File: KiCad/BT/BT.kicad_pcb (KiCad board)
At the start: 4 copper layers, 13.8 x 31.5 mm, 54 parts, among them J1 UJC-HP-3-SMT-TR, J2 2328702-8, J3 Conn_01x05, SW1 Val**, U1 QFN40P120X130X45-6N, U2 SON95P300X300X100-7N-D, U3 STM6601CQ2BDM6F, U4 BMD-350-A-R, U5 UDFN6, U6 UDFN6, U7 UDFN6, Y1 ECS-.327-7-34R-TR

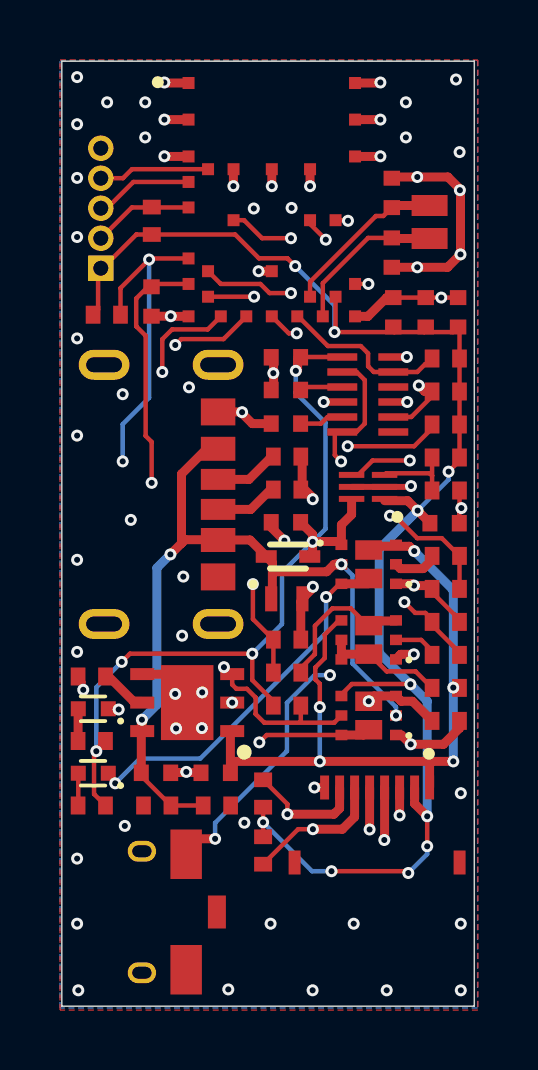
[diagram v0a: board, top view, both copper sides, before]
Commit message: minor updates
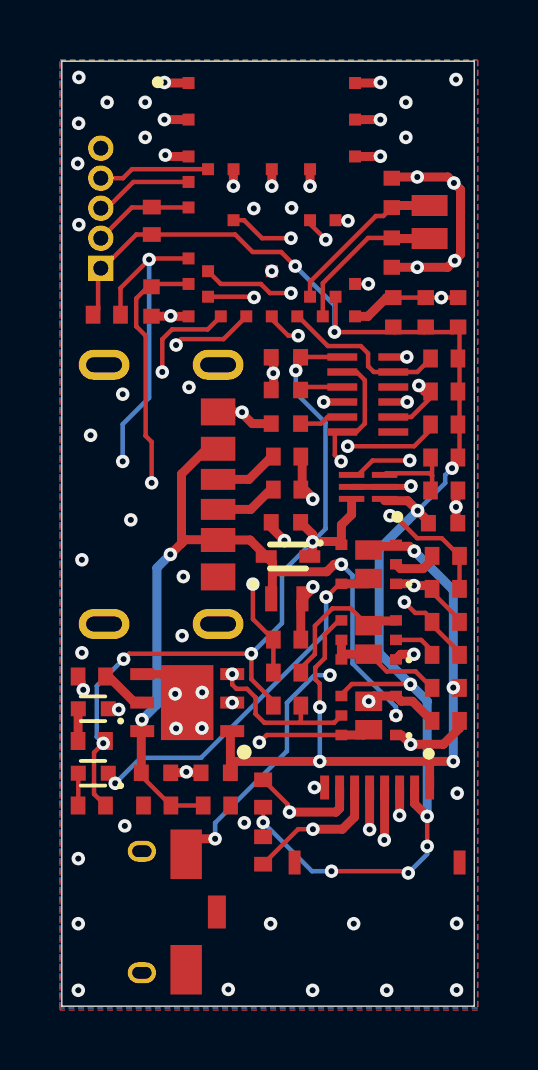
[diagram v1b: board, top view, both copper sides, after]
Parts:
- moved R10 0.05 mm to (107.5, 59.4)
- moved R20 0.05 mm to (107.5, 60.5)
- moved R3 0.05 mm to (107.5, 61.6)
- moved R4 0.05 mm to (107.5, 62.7)
- moved R9 0.05 mm to (107.5, 58.3)
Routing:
- net XSHUT2: track 24.6 -> 24.0 mm
- net GND: track 40.7 -> 40.2 mm, vias 69 -> 67

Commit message: updated
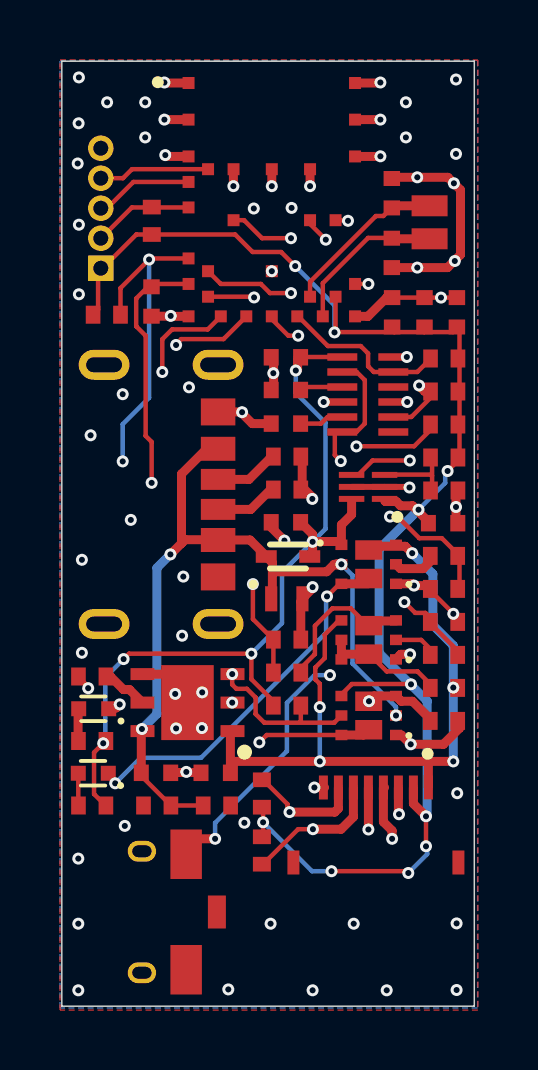
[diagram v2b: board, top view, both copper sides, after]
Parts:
- moved R13 0.06 mm to (107.5, 69.3)
- moved R16 0.06 mm to (107.5, 67.1)
- moved R22 0.06 mm to (107.5, 70.4)
- moved R24 0.06 mm to (107.5, 64.9)
- moved R25 0.06 mm to (107.5, 68.2)
- moved R26 0.06 mm to (107.5, 66.0)
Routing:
- net GND: track 40.2 -> 40.1 mm, vias 67 -> 70
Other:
- board text added: "BT_v6.1"
- board text removed: "BT_v6.0"
